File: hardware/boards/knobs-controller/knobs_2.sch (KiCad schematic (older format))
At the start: 11 parts, among them U2 AP7215-33YG-13, U3 ATSAMD21G18A-48

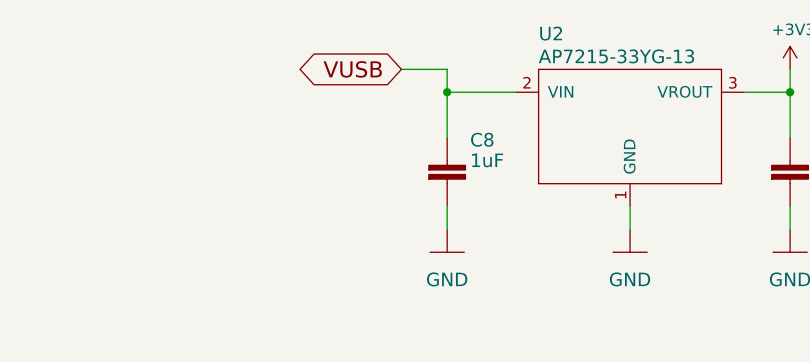
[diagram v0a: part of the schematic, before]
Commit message: routed
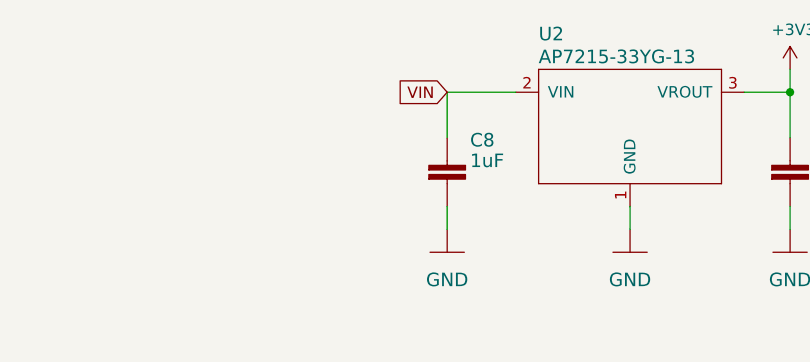
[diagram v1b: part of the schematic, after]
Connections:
- net VUSB renamed VIN
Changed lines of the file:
@@
 	4800 4200 4800 4300
-Wire Wire Line
-	7700 1000 7900 1000
-Wire Wire Line
-	7900 1000 7900 1200
-Wire Wire Line
-	7900 1000 7900 900
-Connection ~ 7900 1000
 Wire Wire Line
 	4200 4900 4200 4800
@@
 Connection ~ 4200 4800
 Connection ~ 4800 4800
-Wire Wire Line
-	6400 1200 6400 1000
-Wire Wire Line
-	6400 1000 6400 900
-Wire Wire Line
-	6400 900  6200 900
-Wire Wire Line
-	6700 1000 6400 1000
-Connection ~ 6400 1000
-Text GLabel 6200 900  0    70   BiDi ~ 0
-VUSB
 $Comp
 L knobs-eagle-import:MK1_ZERO_ATSAMD21G18A-48 U3
@@
 $EndComp
 $Comp
-L power:+3V3 #PWR?
+L power:+3V3 #PWR0115
 U 1 1 5D87F590
 P 4200 3800
-F 0 "#PWR?" H 4200 3650 50  0001 C CNN
+F 0 "#PWR0115" H 4200 3650 50  0001 C CNN
 F 1 "+3V3" H 4215 3973 50  0000 C CNN
 F 2 "" H 4200 3800 50  0001 C CNN
@@
 $EndComp
 $Comp
-L power:+3V3 #PWR?
+L power:+3V3 #PWR0116
 U 1 1 5D8806AC
 P 4800 4200
-F 0 "#PWR?" H 4800 4050 50  0001 C CNN
+F 0 "#PWR0116" H 4800 4050 50  0001 C CNN
 F 1 "+3V3" H 4815 4373 50  0000 C CNN
 F 2 "" H 4800 4200 50  0001 C CNN
@@
 $EndComp
 $Comp
-L power:+3V3 #PWR?
+L power:+3V3 #PWR0117
 U 1 1 5D880E3E
 P 2600 3800
-F 0 "#PWR?" H 2600 3650 50  0001 C CNN
+F 0 "#PWR0117" H 2600 3650 50  0001 C CNN
 F 1 "+3V3" H 2615 3973 50  0000 C CNN
 F 2 "" H 2600 3800 50  0001 C CNN
@@
 $EndComp
 $Comp
-L power:+3V3 #PWR?
+L power:+3V3 #PWR0118
 U 1 1 5D88183D
 P 7900 900
-F 0 "#PWR?" H 7900 750 50  0001 C CNN
+F 0 "#PWR0118" H 7900 750 50  0001 C CNN
 F 1 "+3V3" H 7915 1073 50  0000 C CNN
 F 2 "" H 7900 900 50  0001 C CNN
@@
 $EndComp
 $Comp
-L knobs-eagle-import:GND #GND?
+L knobs-eagle-import:GND #GND0101
 U 1 1 5D883034
 P 2600 4500
-F 0 "#GND?" H 2600 4500 50  0001 C CNN
+F 0 "#GND0101" H 2600 4500 50  0001 C CNN
 F 1 "GND" H 2600 4379 59  0000 C CNN
 F 2 "" H 2600 4500 50  0001 C CNN
@@
 	2600 5300 2600 5200
 $Comp
-L knobs-eagle-import:GND #GND?
+L knobs-eagle-import:GND #GND0102
 U 1 1 5D883C4A
 P 2600 5400
-F 0 "#GND?" H 2600 5400 50  0001 C CNN
+F 0 "#GND0102" H 2600 5400 50  0001 C CNN
 F 1 "GND" H 2600 5279 59  0000 C CNN
 F 2 "" H 2600 5400 50  0001 C CNN
@@
 $EndComp
 $Comp
-L knobs-eagle-import:GND #GND?
+L knobs-eagle-import:GND #GND0103
 U 1 1 5D8841C2
 P 2600 6200
-F 0 "#GND?" H 2600 6200 50  0001 C CNN
+F 0 "#GND0103" H 2600 6200 50  0001 C CNN
 F 1 "GND" H 2600 6079 59  0000 C CNN
 F 2 "" H 2600 6200 50  0001 C CNN
@@
 $EndComp
 $Comp
-L knobs-eagle-import:GND #GND?
+L knobs-eagle-import:GND #GND0104
 U 1 1 5D884790
 P 4200 5900
-F 0 "#GND?" H 4200 5900 50  0001 C CNN
+F 0 "#GND0104" H 4200 5900 50  0001 C CNN
 F 1 "GND" H 4200 5779 59  0000 C CNN
 F 2 "" H 4200 5900 50  0001 C CNN
@@
 $EndComp
 $Comp
-L knobs-eagle-import:GND #GND?
+L knobs-eagle-import:GND #GND0105
 U 1 1 5D884C3C
 P 4200 5400
-F 0 "#GND?" H 4200 5400 50  0001 C CNN
+F 0 "#GND0105" H 4200 5400 50  0001 C CNN
 F 1 "GND" H 4200 5279 59  0000 C CNN
 F 2 "" H 4200 5400 50  0001 C CNN
@@
 $EndComp
 $Comp
-L knobs-eagle-import:GND #GND?
+L knobs-eagle-import:GND #GND0106
 U 1 1 5D88525E
 P 4200 4500
-F 0 "#GND?" H 4200 4500 50  0001 C CNN
+F 0 "#GND0106" H 4200 4500 50  0001 C CNN
 F 1 "GND" H 4200 4379 59  0000 C CNN
 F 2 "" H 4200 4500 50  0001 C CNN
@@
 $EndComp
 $Comp
-L knobs-eagle-import:GND #GND?
+L knobs-eagle-import:GND #GND0107
 U 1 1 5D88564F
 P 6400 1700
-F 0 "#GND?" H 6400 1700 50  0001 C CNN
+F 0 "#GND0107" H 6400 1700 50  0001 C CNN
 F 1 "GND" H 6400 1579 59  0000 C CNN
 F 2 "" H 6400 1700 50  0001 C CNN
@@
 $EndComp
 $Comp
-L knobs-eagle-import:GND #GND?
+L knobs-eagle-import:GND #GND0108
 U 1 1 5D885B2E
 P 7200 1700
-F 0 "#GND?" H 7200 1700 50  0001 C CNN
+F 0 "#GND0108" H 7200 1700 50  0001 C CNN
 F 1 "GND" H 7200 1579 59  0000 C CNN
 F 2 "" H 7200 1700 50  0001 C CNN
@@
 $EndComp
 $Comp
-L knobs-eagle-import:GND #GND?
+L knobs-eagle-import:GND #GND0109
 U 1 1 5D885ECA
 P 7900 1700
-F 0 "#GND?" H 7900 1700 50  0001 C CNN
+F 0 "#GND0109" H 7900 1700 50  0001 C CNN
 F 1 "GND" H 7900 1579 59  0000 C CNN
 F 2 "" H 7900 1700 50  0001 C CNN
@@
 	4100 3900 4200 3900
 $Comp
-L power:+3V3 #PWR?
+L power:+3V3 #PWR0119
 U 1 1 5D88CD3D
 P 2350 5600
-F 0 "#PWR?" H 2350 5450 50  0001 C CNN
+F 0 "#PWR0119" H 2350 5450 50  0001 C CNN
 F 1 "+3V3" H 2365 5773 50  0000 C CNN
 F 2 "" H 2350 5600 50  0001 C CNN
@@
 Wire Wire Line
 	2700 4300 2600 4300
+Wire Wire Line
+	7700 1000 7900 1000
+Wire Wire Line
+	7900 1000 7900 900
+Wire Wire Line
+	7900 1000 7900 1200
+Connection ~ 7900 1000
+Wire Wire Line
+	6400 1200 6400 1000
+Wire Wire Line
+	6400 1000 6700 1000
+Text GLabel 6400 1000 0    50   Input ~ 0
+VIN
 $EndSCHEMATC
